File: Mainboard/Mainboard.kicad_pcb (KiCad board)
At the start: 4 copper layers, 106.1 x 132 mm, 128 parts, among them IC1 REF102AU_2K5, IC4 DAC8814IBDBT, J1 5745782-6, J2 5745782-6, J3 5745782-6, J4 Conn_01x02_Pin, J5 Conn_01x02_Pin, J6 Conn_01x02_Pin, U1 Teensy4.0, U10 TL072, U11 ADG419BR, U12 ADG419BR, U2 TL072, U3 TL072, U4 TL072, U5 TL074, U6 TL074, U7 ADG419BR, U8 LTC2326CMS-16-PBF, U9 LT1469CS8-TRPBF

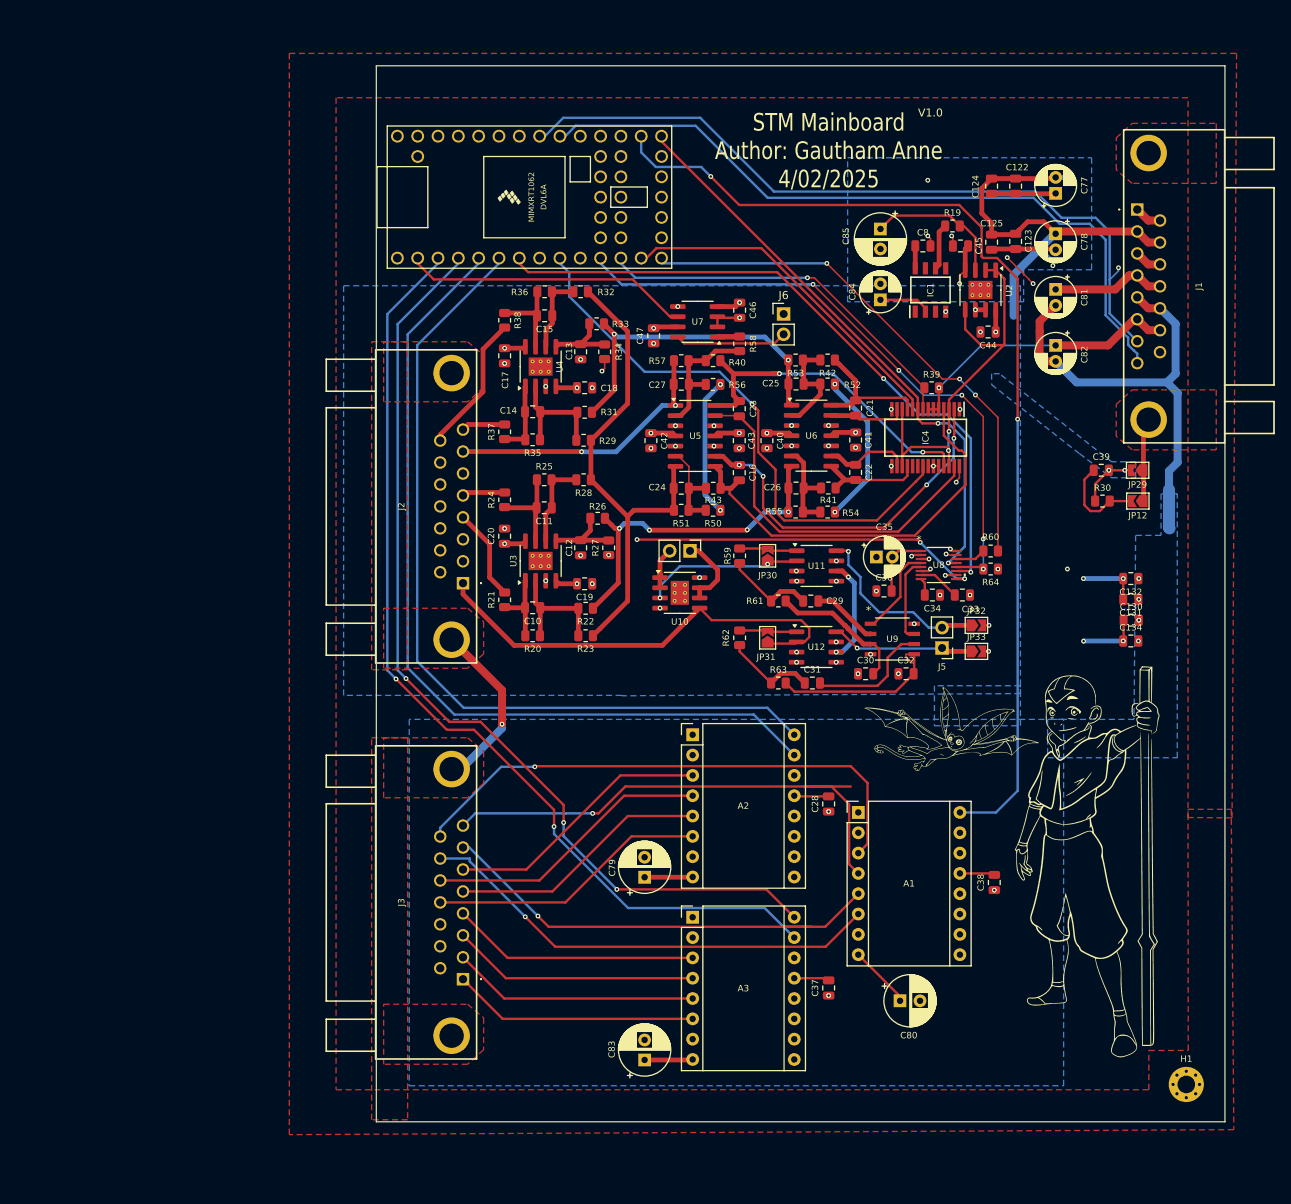
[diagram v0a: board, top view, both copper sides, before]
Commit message: cad update
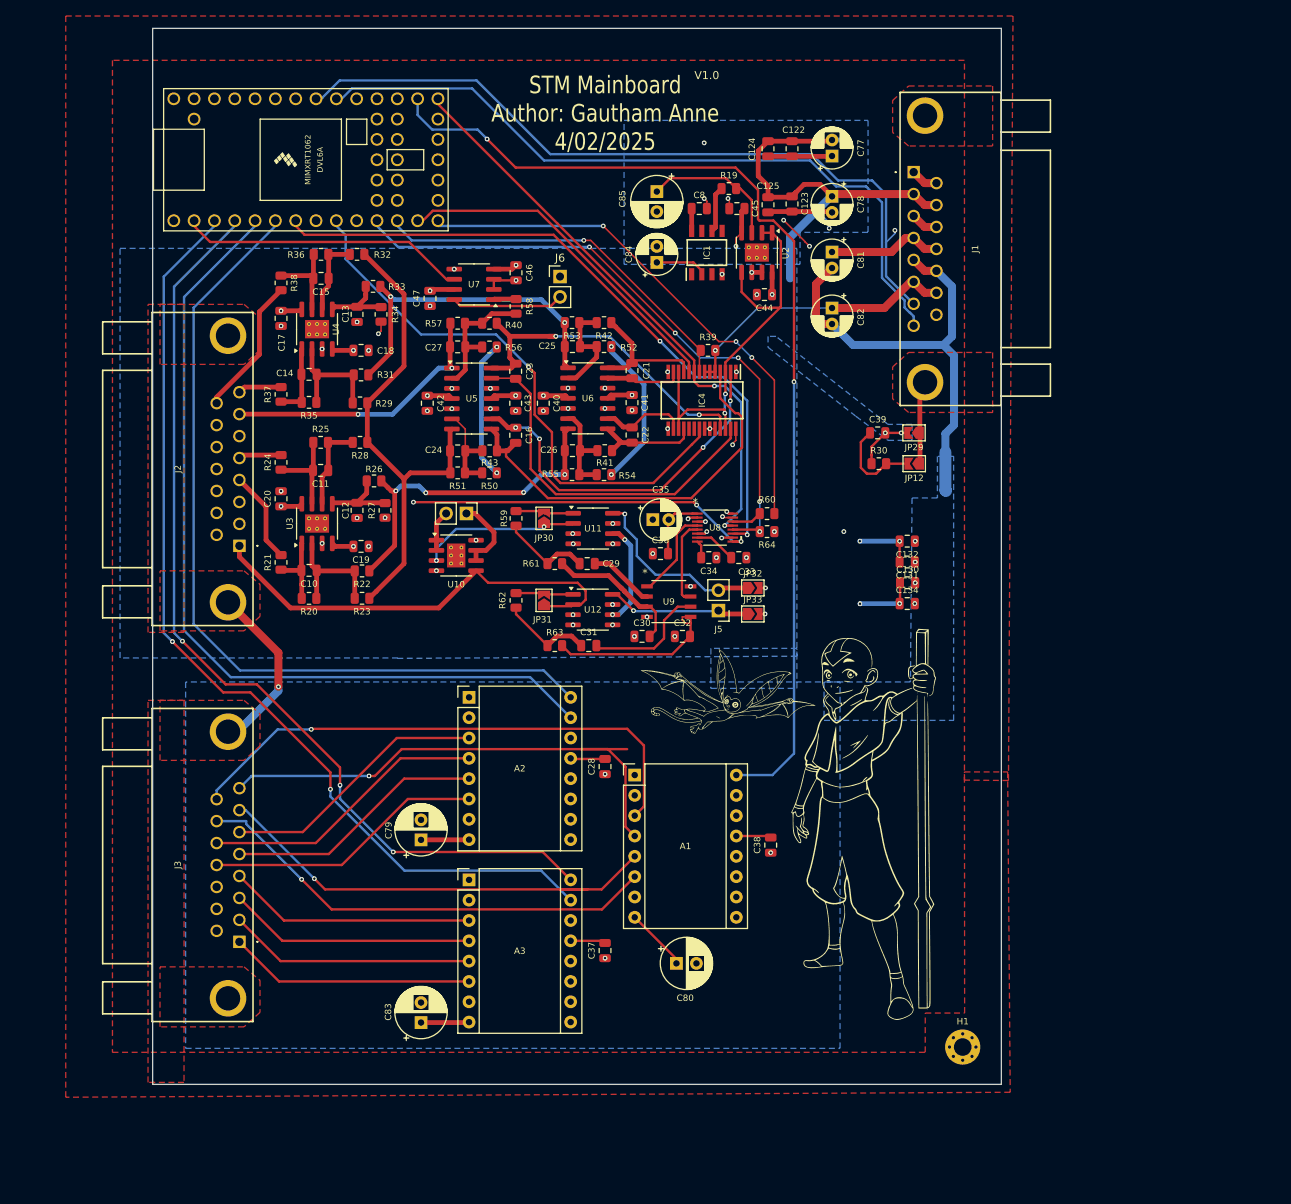
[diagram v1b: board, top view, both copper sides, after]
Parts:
- moved A3 28.3 mm to (130.7, 129.3)
- moved C134 28.3 mm to (185.4, 94.7)
- moved C24 28.3 mm to (129.3, 75.6)
- moved C25 28.3 mm to (143.6, 62.6)
- moved C26 28.3 mm to (143.6, 75.6)
- moved C27 28.3 mm to (129.3, 62.6)
- moved C37 28.3 mm to (147.7, 138.1)
- moved C38 28.3 mm to (168.4, 124.9)
- moved C80 28.3 mm to (156.6, 139.7)
- moved J1 28.3 mm to (186.3, 40.8)
- moved J4 28.3 mm to (130.3, 83.5)
- moved J5 28.3 mm to (161.8, 95.6)
- moved R40 28.3 mm to (133.2, 59.7)
- moved R41 28.3 mm to (147.6, 75.6)
- moved R43 28.3 mm to (133.3, 75.6)
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
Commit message: updates!
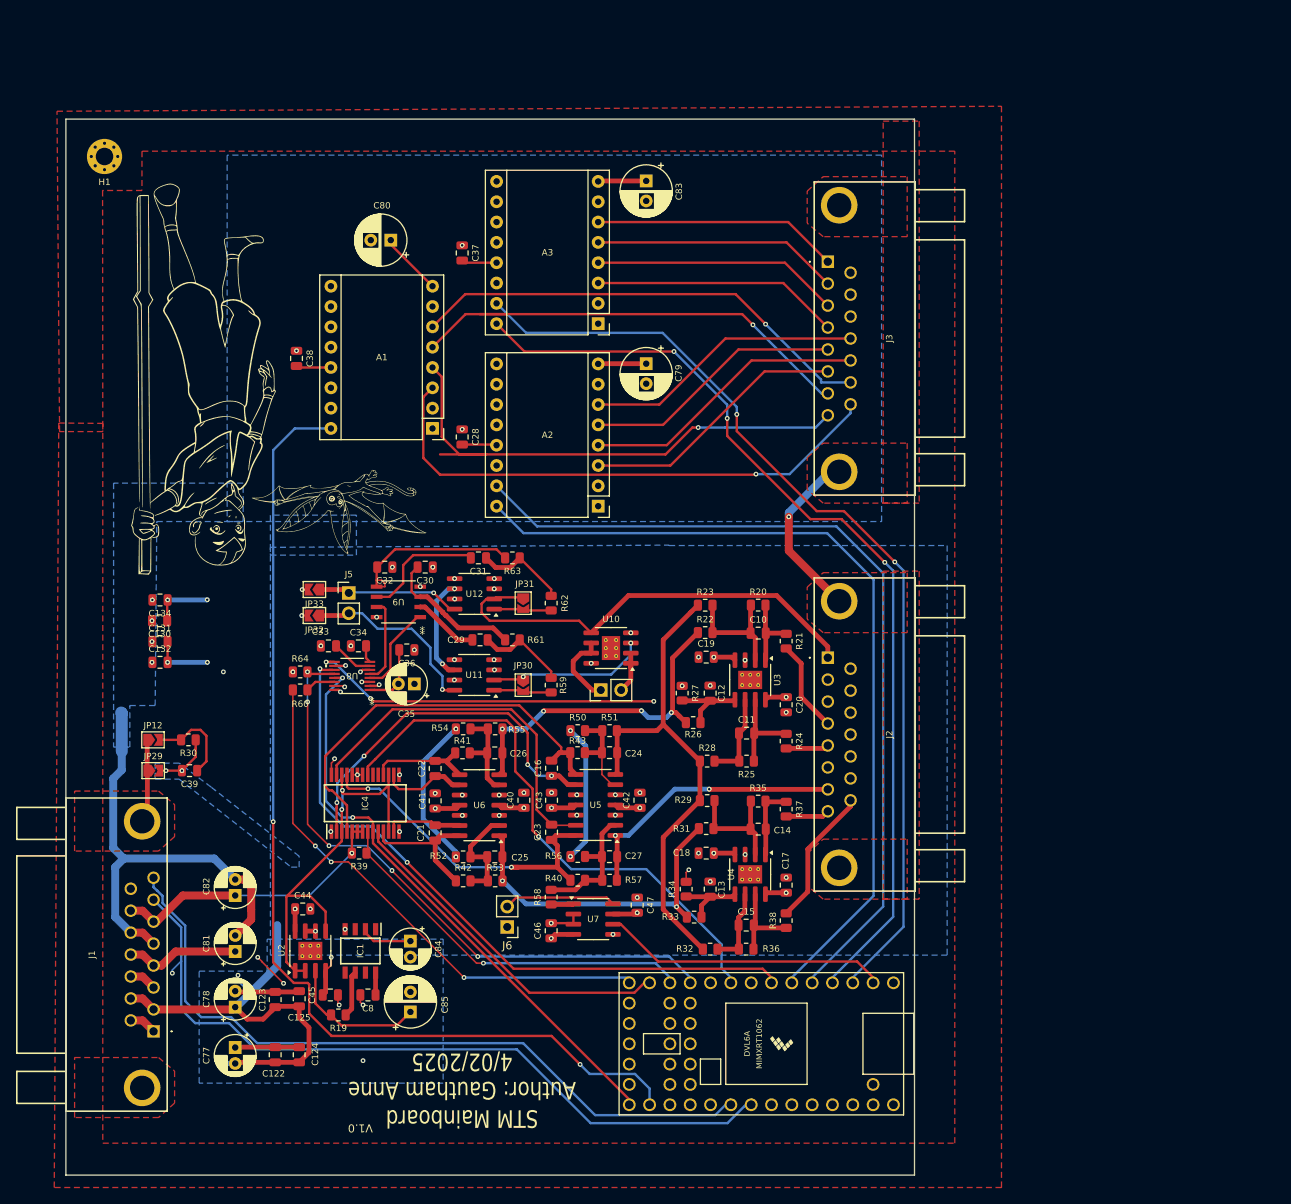
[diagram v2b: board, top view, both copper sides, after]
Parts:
- moved H1 154.6 mm to (85.1, 38.8), turned to 180 degrees
- moved J1 143.4 mm to (91.2, 148.2), turned to -90 degrees
- moved C77 134.1 mm to (101.4, 150.2), turned to -90 degrees
- moved C122 130.4 mm to (106.4, 151.1), turned to -90 degrees
- moved C124 127.5 mm to (109.4, 151.1), turned to -90 degrees
- moved C78 125.8 mm to (101.4, 145.2), turned to 90 degrees
- moved U1 124.3 mm to (167.2, 149.8), turned to 180 degrees
- moved C123 118.6 mm to (106.4, 144.2), turned to 90 degrees
- moved C125 115.3 mm to (109.4, 144.1), turned to 90 degrees
- moved C81 114.9 mm to (101.4, 138.2), turned to 90 degrees
- moved R19 114.2 mm to (114.3, 146.1), turned to 180 degrees
- moved J3 112.4 mm to (175.5, 52.0), turned to 90 degrees
- moved C45 110.7 mm to (113.3, 143.6), turned to 180 degrees
- moved C83 108.9 mm to (152.8, 41.9), turned to -90 degrees
- moved C85 107.1 mm to (123.3, 145.8), turned to 90 degrees
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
